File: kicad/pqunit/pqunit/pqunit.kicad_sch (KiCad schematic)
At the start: 5 parts, among them IC1 ATGM332D-5N31, J1 PQ9_Socket, U1 ATmega328PB-A, U2 Ai-Thinker-Ra-02

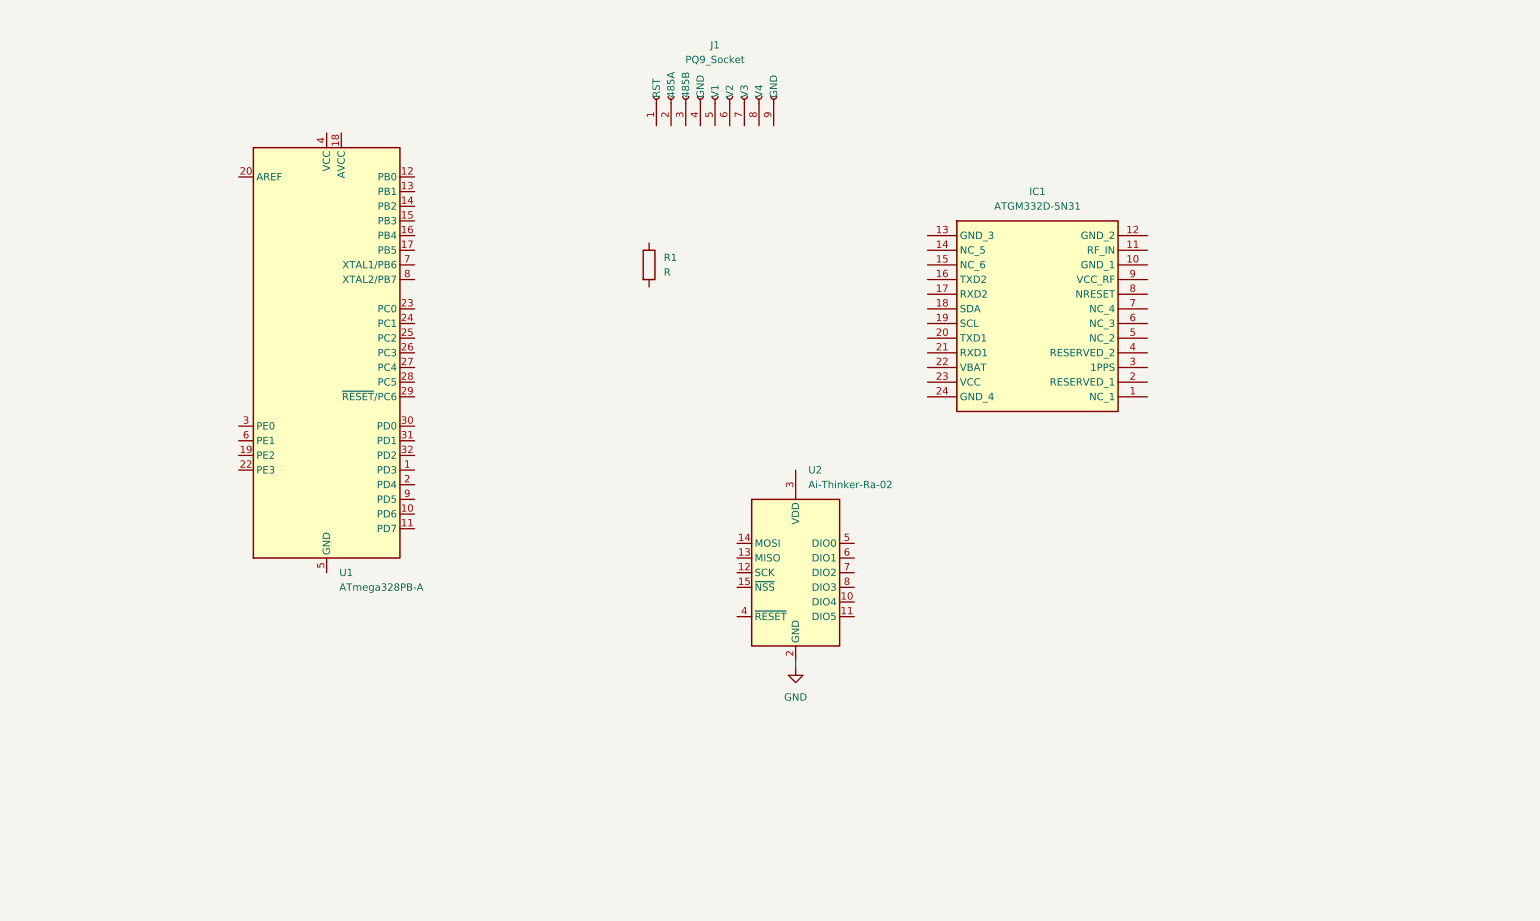
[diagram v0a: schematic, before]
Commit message: Worked on schematics
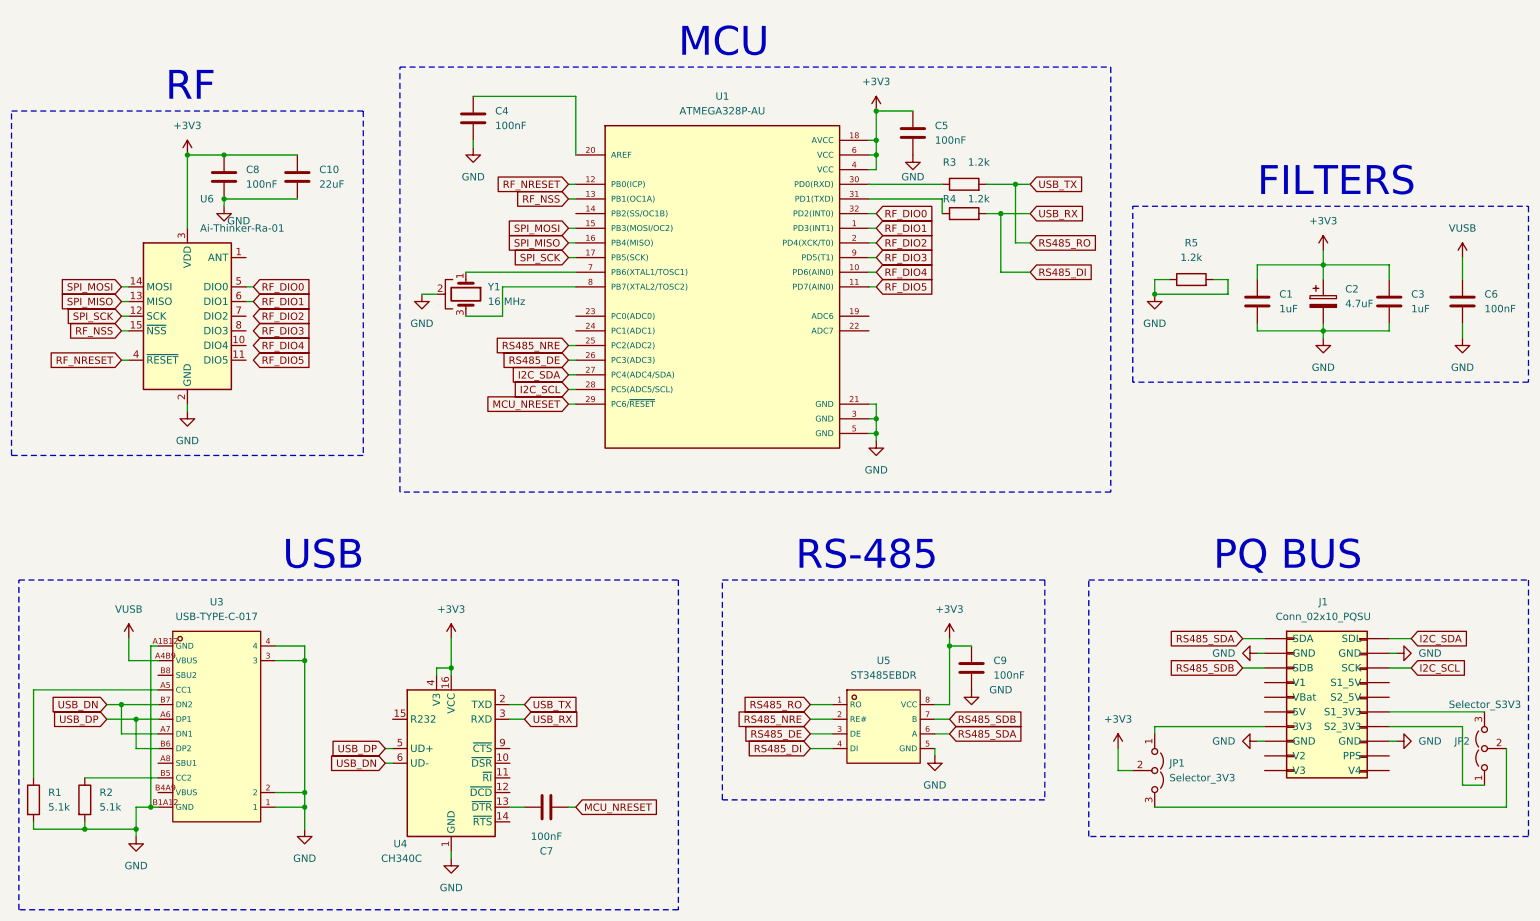
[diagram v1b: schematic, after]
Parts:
- removed IC1: ATGM332D-5N31, ATGM332D5N31, symbol ATGM332D-5N31:ATGM332D-5N31
- removed J1: PQ9_Socket, symbol Connector:Conn_01x09_Socket
- removed U1: ATmega328PB-A, Package_QFP:TQFP-32_7x7mm_P0.8mm, symbol MCU_Microchip_ATmega:ATmega328PB-A
- removed U2: Ai-Thinker-Ra-02, RF_Module:Ai-Thinker-Ra-01-LoRa, symbol RF_Module:Ai-Thinker-Ra-02
- added C1, C3: 1uF, CL21B105KAFNNNE (1uF):CL21B105KAFNNNE, symbol Device:C
- added C10: 22uF, C3216X5R1V226MTJ00E (22uF):C3216X5R1V226MTJ00E, symbol Device:C
- added C2: 4.7uF, 0805X475K160NT (4.7uF):0805X475K160NT, symbol Device:C_Polarized
- added C4, C5, C6, C7, C8, C9: 100nF, 06035C104K4Z2A (100nF):06035C104K4Z2A, symbol Device:C
- added J1: Conn_02x10_PQSU, Connector_PinSocket_2.54mm:PinSocket_2x10_P2.54mm_Vertical, symbol Connector_Generic:Conn_02x10_Top_Bottom
- added JP1: Selector_3V3, Jumper:SolderJumper-3_P1.3mm_Open_Pad1.0x1.5mm_NumberLabels, symbol Jumper:Jumper_3_Open
- added JP2: Selector_S3V3, Jumper:SolderJumper-3_P1.3mm_Open_Pad1.0x1.5mm_NumberLabels, symbol Jumper:Jumper_3_Open
- added R2: 5.1k, CR1206J40512G:CR1206J40122G, symbol Device:R
- added R3, R4, R5: 1.2k, CR1206J40122G:CR1206J40122G, symbol Device:R
- added U1: ATMEGA328P-AU, QFP80P900X900X120-32N, symbol ATMEGA328P-AU:ATMEGA328P-AU
- added U3: USB-TYPE-C-017, USB-TYPE-C-017:USB-TYPE-C-SMD_C9900008089, symbol USB-TYPE-C-017:USB-TYPE-C-017
- added U4: CH340C, Package_SO:SOIC-16_3.9x9.9mm_P1.27mm, symbol Interface_USB:CH340C
- added U5: ST3485EBDR, ST3485EBDR:ST3485EBDR, symbol ST3485EBDR:ST3485EBDR
- added U6: Ai-Thinker-Ra-01, RF_Module:Ai-Thinker-Ra-01-LoRa, symbol RF_Module:Ai-Thinker-Ra-01
- added Y1: 16 MHz, CSTCE16M0V53-R0:CSTCE16M0V53-R0, symbol Device:Crystal_GND2
- R1: value R -> 5.1k; footprint (none) -> CR1206J40512G:CR1206J40122G
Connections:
- net GND: now also R1.2, C1.2, C10.2, C2.2, C3.2, C4.2, C5.2, C6.2, C8.2, C9.2, J1.12 (GND), J1.18 (GND), J1.2 (GND), J1.8 (GND), R2.2, R5.1, R5.2, U1.21 (GND), U1.3 (GND), U1.5 (GND), U3.1, U3.2, U3.3, U3.4, U3.A1B12 (GND), U3.B1A12 (GND), U4.1 (GND), U5.5 (GND), U6.16 (GND), U6.2 (GND), U6.9 (GND), Y1.2
- net at R1.1: now also U3.A5 (CC1)
- new net: C7.2, U4.13 (~{DTR})
- new net: R3.1, U1.30 (PD0(RXD))
- new net: R2.1, U3.B5 (CC2)
- new net: J1.17 (S2_3V3), JP2.1 (A)
- new net: JP1.3 (B), JP2.2 (C)
- new net: J1.16 (S1_3V3), JP2.3 (B)
- new net: J1.7 (3V3), JP1.1 (A)
- new net: U1.7 (PB6(XTAL1/TOSC1)), Y1.1
- new net: U1.8 (PB7(XTAL2/TOSC2)), Y1.3
- new net: R4.1, U1.31 (PD1(TXD))
- new net: C4.1, U1.20 (AREF)
- new net +3V3: C1.1, C10.1, C2.1, C3.1, C5.1, C8.1, C9.1, JP1.2 (C), U1.18 (AVCC), U1.4 (VCC), U1.6 (VCC), U4.16 (VCC), U4.4 (V3), U5.8 (VCC), U6.3 (VDD)
- new net I2C_SCL: J1.13 (SCK), U1.28 (PC5(ADC5/SCL))
- new net I2C_SDA: J1.11 (SDL), U1.27 (PC4(ADC4/SDA))
- new net MCU_NRESET: C7.1, U1.29 (PC6/~{RESET})
- new net RF_DIO0: U1.32 (PD2(INT0)), U6.5 (DIO0)
- new net RF_DIO1: U1.1 (PD3(INT1)), U6.6 (DIO1)
- new net RF_DIO2: U1.2 (PD4(XCK/T0))
- new net RF_DIO3: U1.9 (PD5(T1))
- new net RF_DIO4: U1.10 (PD6(AIN0))
- new net RF_DIO5: U1.11 (PD7(AIN0))
- new net RF_NRESET: U1.12 (PB0(ICP)), U6.4 (~{RESET})
- new net RF_NSS: U1.13 (PB1(OC1A)), U6.15 (~{NSS})
- new net RS485_DE: U1.26 (PC3(ADC3)), U5.3 (DE)
- new net RS485_DI: R4.2, U4.3 (RXD), U5.4 (DI)
- new net RS485_NRE: U1.25 (PC2(ADC2)), U5.2 (RE#)
- new net RS485_RO: R3.2, U4.2 (TXD), U5.1 (RO)
- new net RS485_SDA: J1.1 (SDA), U5.6 (A)
- new net RS485_SDB: J1.3 (SDB), U5.7 (B)
- new net SPI_MISO: U1.16 (PB4(MISO)), U6.13 (MISO)
- new net SPI_MOSI: U1.15 (PB3(MOSI/OC2)), U6.14 (MOSI)
- new net SPI_SCK: U1.17 (PB5(SCK)), U6.12 (SCK)
- new net USB_DN: U3.A7 (DN1), U3.B7 (DN2), U4.6 (UD-)
- new net USB_DP: U3.A6 (DP1), U3.B6 (DP2), U4.5 (UD+)
- new net VUSB: C6.1, U3.A4B9 (VBUS)
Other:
- note added: "FILTERS"
- note added: "MCU"
- note added: "PQ BUS"
- note added: "RF"
- note added: "RS-485"
- note added: "USB"
